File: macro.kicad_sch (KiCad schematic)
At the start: 68 parts, among them J1 Conn_01x01_Male, J2 Conn_01x01_Male, J3 Conn_01x01_Male, Q1 BSS138, SW1 RotaryEncoder_Switch, SW2 SW_Push, U1 AP2112K-3.3, U2 W25Q128JVPIQ, U3 RP2040, Y1 12MHz

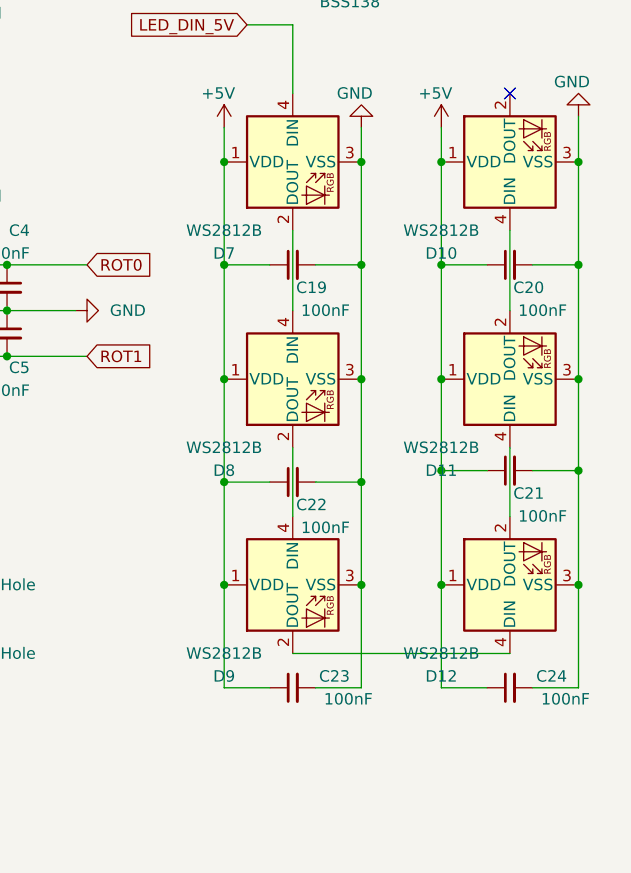
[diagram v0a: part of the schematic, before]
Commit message: Update
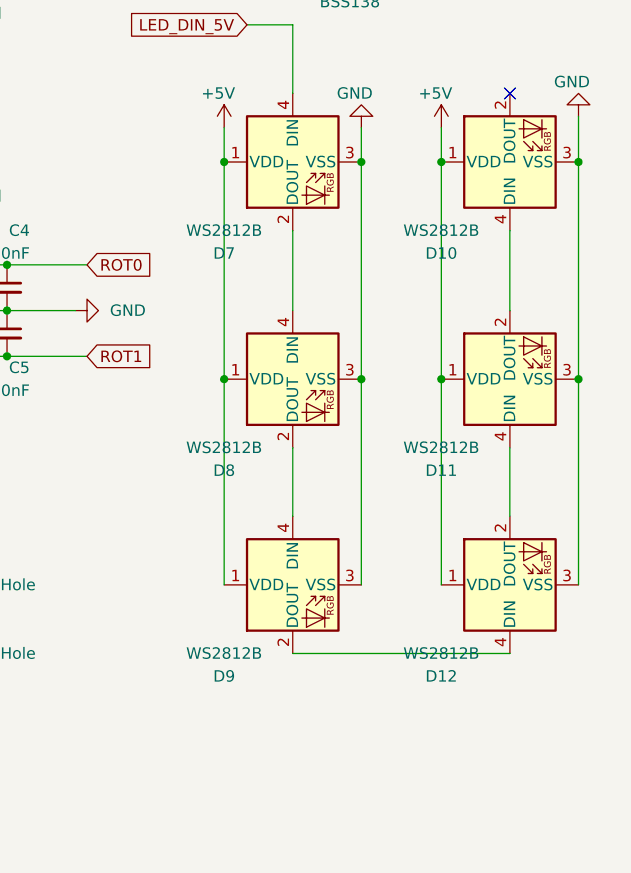
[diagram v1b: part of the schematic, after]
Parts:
- removed C19, C20, C21, C22, C23, C24: 100nF, Capacitor_SMD:C_0402_1005Metric, symbol Device:C_Small
